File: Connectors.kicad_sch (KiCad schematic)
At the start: 68 parts, among them J1 SM05B-GHS-TB, J10 Header1x3Pin, J15 SM07B-GHS-TB, J16 SM02B-GHS-TB, J18 USB_C_Receptacle, J4 SM05B-GHS-TB, J6 SM05B-GHS-TB, J6 SM07B-GHS-TB, J8 Header1x3Pin

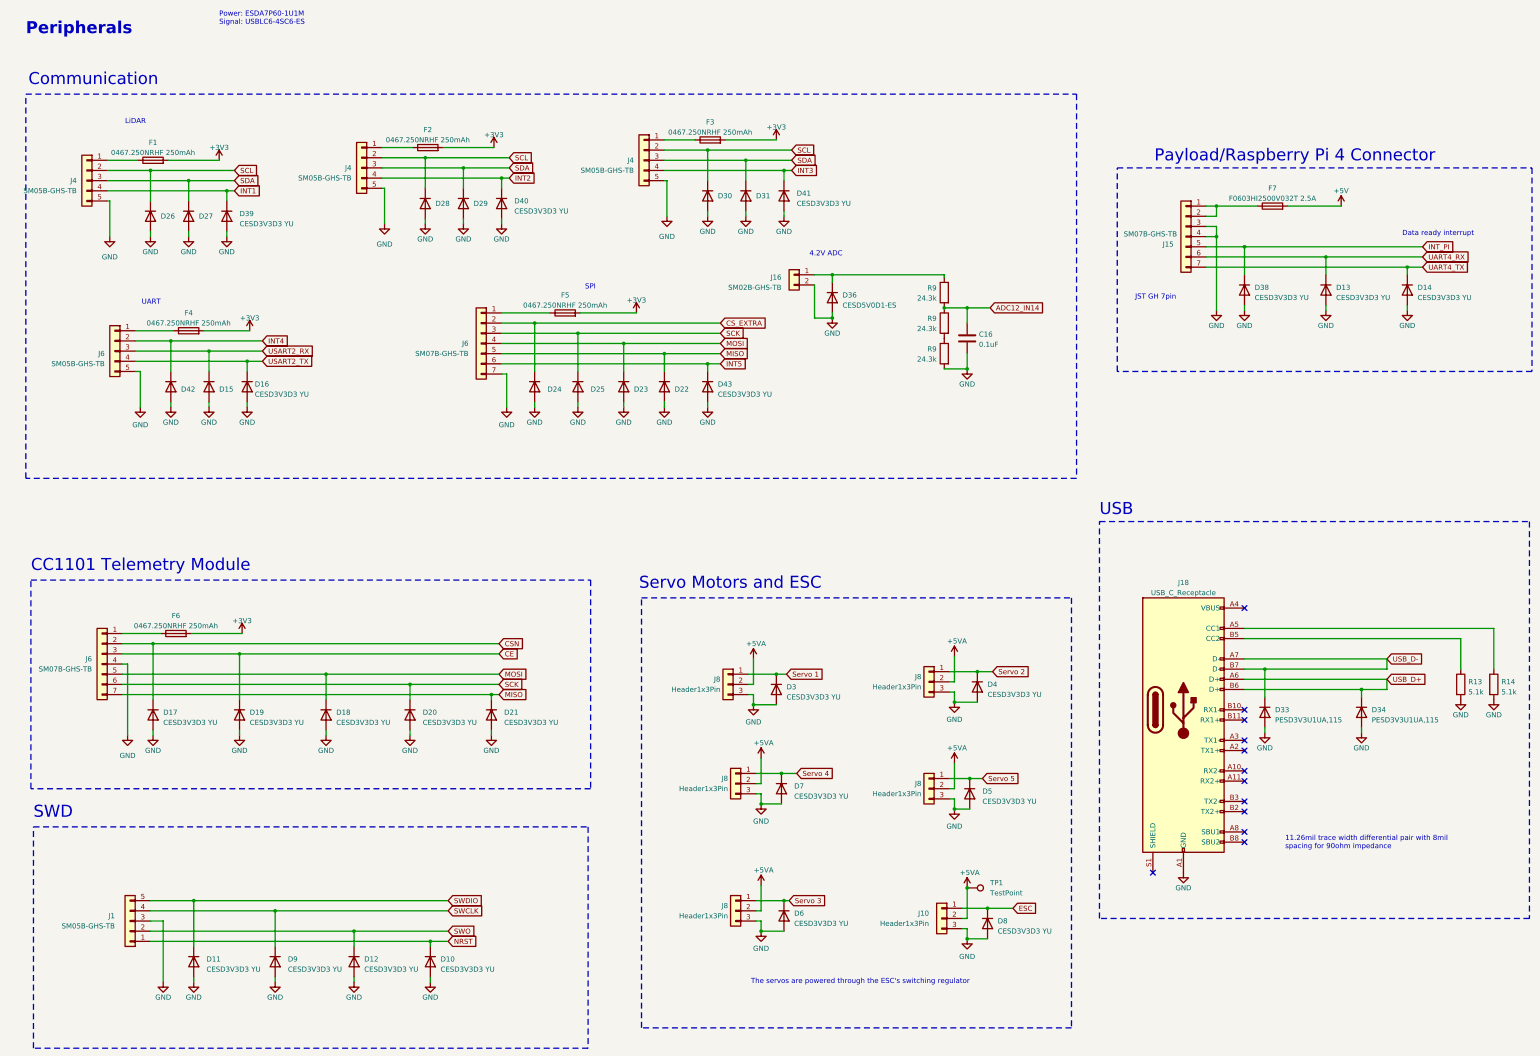
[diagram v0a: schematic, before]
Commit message: Add files via upload
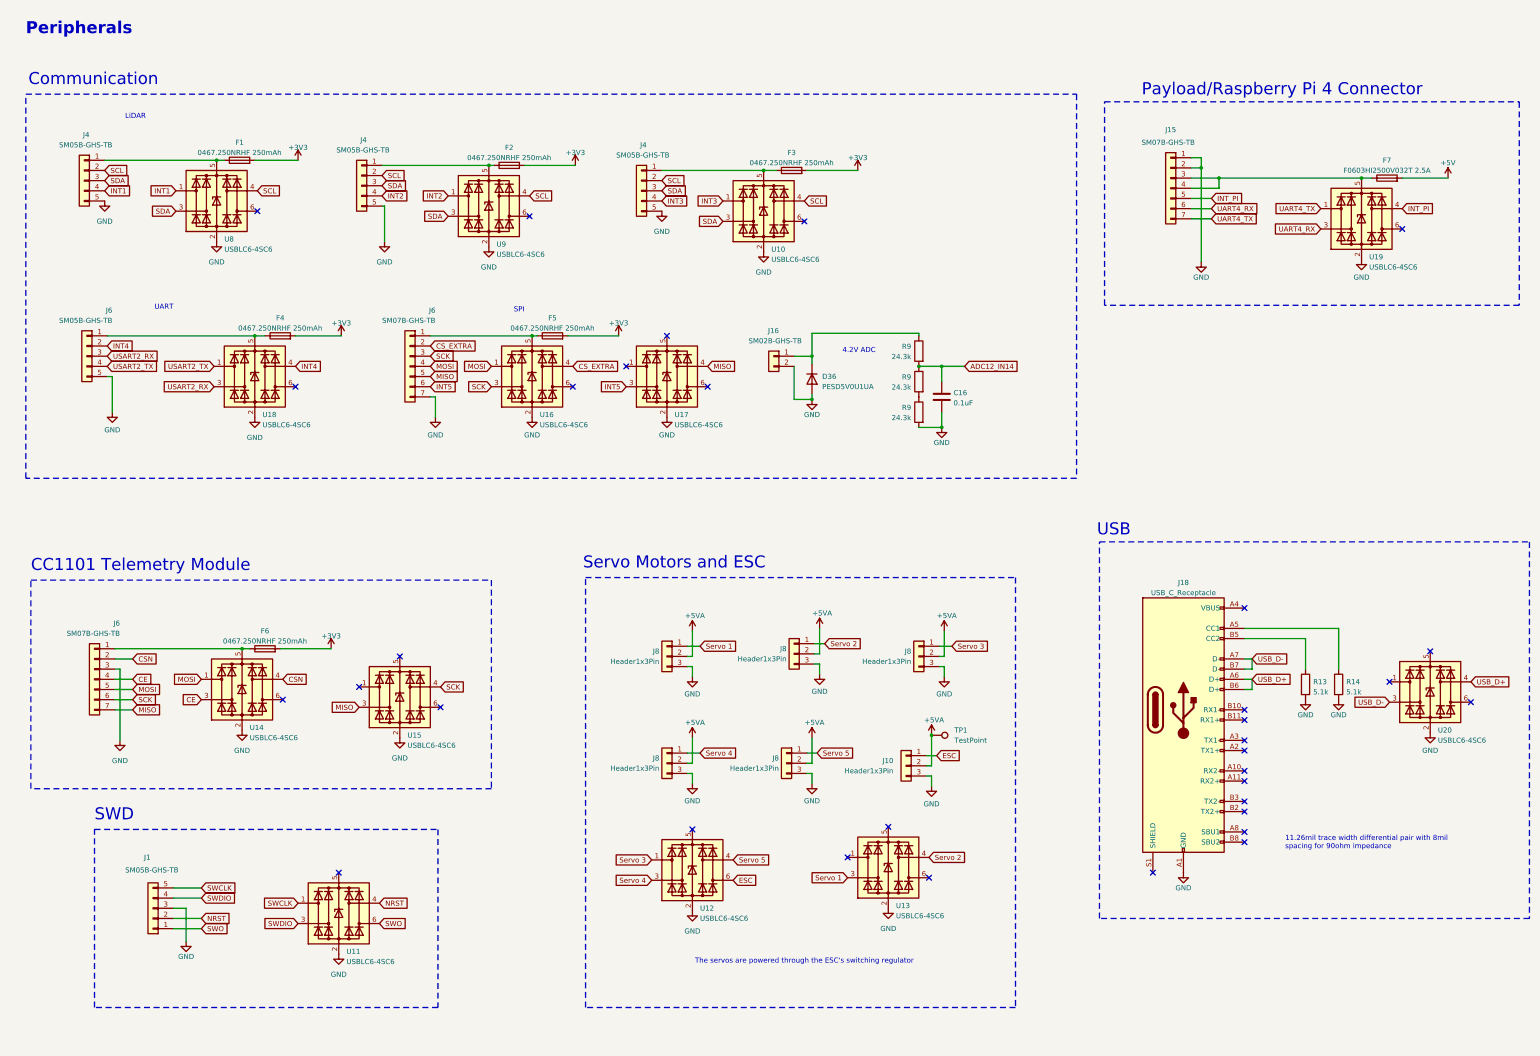
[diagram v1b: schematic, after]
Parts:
- removed D10, D11, D12, D13, D14, D15, D16, D17, D18, D19, D20, D21, D22, D23, D24, D25, D26, D27, D28, D29, D3, D30, D31, D38, D39, D4, D40, D41, D42, D43, D5, D6, D7, D8, D9: CESD3V3D3 YU, Diode_SMD:D_SOD-323, symbol Device:D
- removed D33, D34: PESD3V3U1UA,115, Diode_SMD:D_SOD-323, symbol Device:D
- added U10, U11, U12, U13, U14, U15, U16, U17, U18, U19, U20, U8, U9: USBLC6-4SC6, Package_TO_SOT_SMD:SOT-23-6, symbol Power_Protection:USBLC6-4SC6
- D36: value CESD5V0D1-ES -> PESD5V0U1UA
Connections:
- net CE: now also J6.4 (Pin_4), U14.3 (I/O2); no longer J6.3 (Pin_3)
- net CSN: now also U14.4 (I/O3)
- net CS_EXTRA: now also U16.4 (I/O3)
- net ESC: now also U12.6 (I/O4)
- net GND: now also J15.1 (Pin_1), J15.2 (Pin_2), J6.3 (Pin_3), U10.2 (GND), U11.2 (GND), U12.2 (GND), U13.2 (GND), U14.2 (GND), U15.2 (GND), U16.2 (GND), U17.2 (GND), U18.2 (GND), U19.2 (GND), U20.2 (GND), U8.2 (GND), U9.2 (GND); no longer J15.3 (Pin_3), J15.4 (Pin_4), J6.4 (Pin_4)
- net INT1: now also U8.1 (I/O1)
- net INT2: now also U9.1 (I/O1)
- net INT3: now also U10.1 (I/O1)
- net INT4: now also U18.4 (I/O3)
- net INT5: now also U17.3 (I/O2)
- net INT_PI: now also U19.4 (I/O3)
- net MISO: now also U15.3 (I/O2), U17.4 (I/O3)
- net MOSI: now also U14.1 (I/O1), U16.1 (I/O1)
- net NRST: now also J1.2 (Pin_2), U11.4 (I/O3); no longer J1.1 (Pin_1)
- net SCK: now also U15.4 (I/O3), U16.3 (I/O2)
- net SCL: now also U10.4 (I/O3), U8.4 (I/O3), U9.4 (I/O3)
- net SDA: now also U10.3 (I/O2), U8.3 (I/O2), U9.3 (I/O2)
- net SWCLK: now also J1.5 (Pin_5), U11.1 (I/O1); no longer J1.4 (Pin_4)
- net SWDIO: now also J1.4 (Pin_4), U11.3 (I/O2); no longer J1.5 (Pin_5)
- net SWO: now also J1.1 (Pin_1), U11.6 (I/O4); no longer J1.2 (Pin_2)
- net Servo 1: now also U13.3 (I/O2)
- net Servo 2: now also U13.4 (I/O3)
- net Servo 3: now also U12.1 (I/O1)
- net Servo 4: now also U12.3 (I/O2)
- net Servo 5: now also U12.4 (I/O3)
- net UART4_RX: now also U19.3 (I/O2)
- net UART4_TX: now also U19.1 (I/O1)
- net USART2_RX: now also U18.3 (I/O2)
- net USART2_TX: now also U18.1 (I/O1)
- net USB_D+: now also U20.4 (I/O3)
- net USB_D-: now also U20.3 (I/O2)
- net at F5.1, J6.1 (Pin_1): now also U16.5 (VBUS)
- net at F3.1, J4.1 (Pin_1): now also U10.5 (VBUS)
- net at F1.1, J4.1 (Pin_1): now also U8.5 (VBUS)
- net at F6.1, J6.1 (Pin_1): now also U14.5 (VBUS)
- net at F4.1, J6.1 (Pin_1): now also U18.5 (VBUS)
- net at F2.1, J4.1 (Pin_1): now also U9.5 (VBUS)
- new net: F7.1, J15.3 (Pin_3), J15.4 (Pin_4), U19.5 (VBUS)
- no-connect marks 12 -> 33
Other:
- note removed: "Data ready interrupt"
- note removed: "JST GH 7pin"
- note removed: "Power: ESDA7P60-1U1M Signal: USBLC6-4SC6-ES"
- moved on the sheet: C16, D36, F1, F2, F3, F4, F5, F6, F7, J1, J10, J15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

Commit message: Add files via upload
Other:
- note added: "ADC"
- note added: "I2C"
- note removed: "Communication"
- moved on the sheet: C16, D36, F1, F2, F3, F4, F5, F7, J1, J10, J15, J16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
